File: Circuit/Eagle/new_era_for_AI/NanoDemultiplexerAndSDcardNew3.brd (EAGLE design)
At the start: 94 x 70 mm, 22 parts

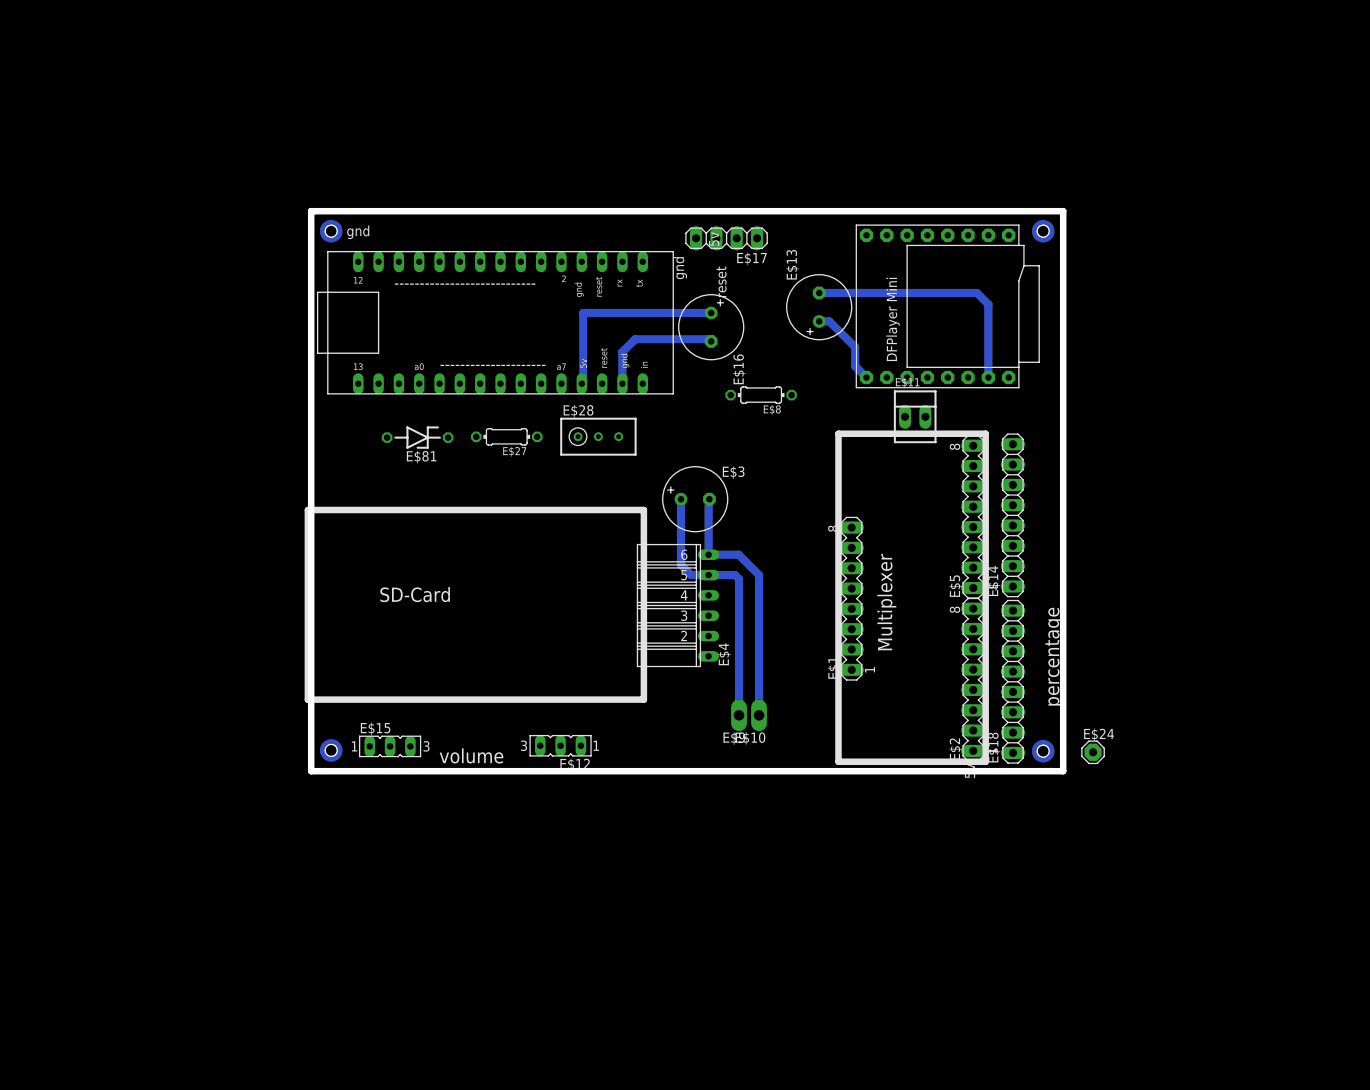
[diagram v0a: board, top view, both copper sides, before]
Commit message: .
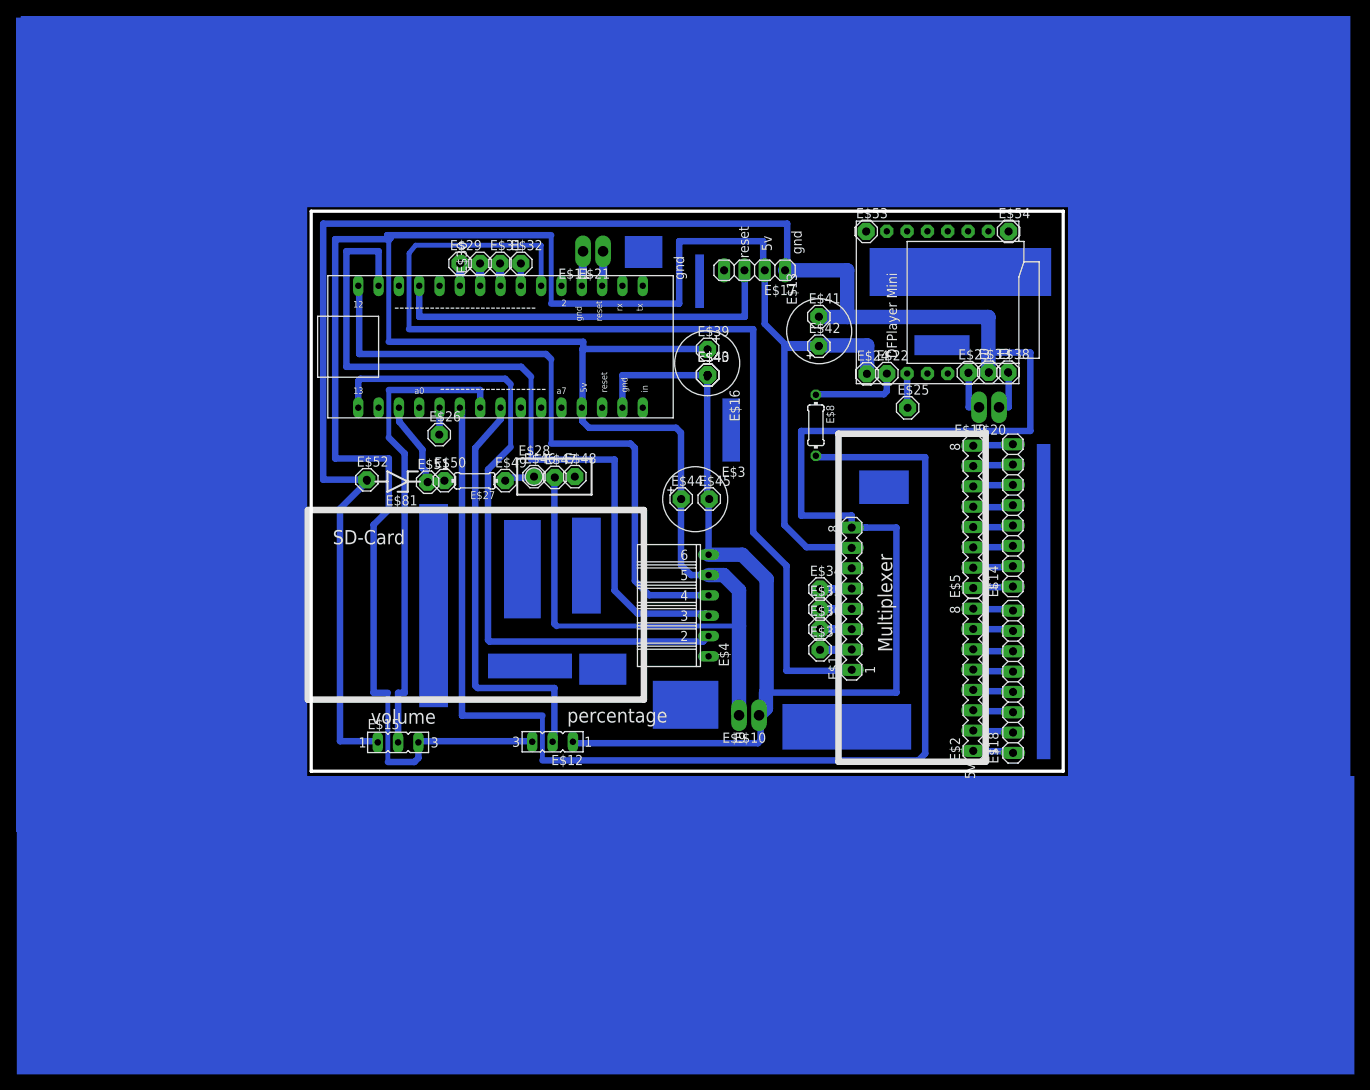
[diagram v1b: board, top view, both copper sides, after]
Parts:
- added E$19, E$20, E$21: (no value), testpad:P1-13Y
- added E$22, E$23, E$25, E$26, E$29, E$30, E$31, E$32, E$33, E$34, E$35, E$36, E$37, E$38, E$39, E$40, E$41, E$42, E$43, E$44, E$45, E$46, E$47, E$48, E$49, E$50, E$51, E$52, E$53, E$54: (no value), solpad:MCS10B
- E$11: device con-molex:22-23-2021 -> testpad:P1-13Y
- moved E$24 55.1 mm to (75.5, 51.7)
- moved E$11 46.4 mm to (40.0, 67.0), turned to 180 degrees
- moved E$8 7.81 mm to (69.1, 45.2), turned to 270 degrees
- moved E$28 7.43 mm to (36.4, 38.8)
- moved E$27 6.80 mm to (26.4, 38.3)
- moved E$81 6.04 mm to (16.8, 38.2)
- moved E$17 5.32 mm to (61.4, 64.6)
- moved E$16 4.53 mm to (55.5, 53.0)
- moved E$13 3.00 mm to (69.5, 57.0)
- moved E$7 3.00 mm to (29.7, 55.1)
- moved E$12 1.12 mm to (33.6, 5.68)
- moved E$15 1.12 mm to (19.4, 5.60)
- moved E$6 0.50 mm to (84.3, 60.6)
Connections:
- new net SPK3: E$11.TP, E$7.P$24
- new net SPK4: E$21.TP, E$7.P$25
- net S0: now also E$32.MP, E$34.MP
- net S1: now also E$31.MP, E$35.MP
- net S2: now also E$30.MP, E$36.MP
- net S3: now also E$29.MP, E$37.MP
- net SPK1: now also E$19.TP; no longer E$11.1
- net SPK2: now also E$20.TP; no longer E$11.2
- net TX: now also E$25.MP, E$26.MP
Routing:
- net 5V: track 68.4 -> 384.5 mm
- net GND: track 78.6 -> 376.8 mm
- net S$10: track 0.00 -> 153.3 mm
- net SIGN: track 0.00 -> 127.2 mm
- net MOSI: track 0.00 -> 96.6 mm
- net SCK: track 0.00 -> 83.9 mm
- net MISO: track 0.00 -> 80.6 mm
- net VOLUME-CONTROL: track 0.00 -> 59.3 mm
- net S$4: track 0.00 -> 52.8 mm
- net RESET: track 0.00 -> 50.4 mm
- net S$2: track 0.00 -> 12.7 mm
- net RX: track 0.00 -> 11.3 mm
- net TX: track 0.00 -> 7.70 mm
- net S1: track 0.00 -> 6.78 mm
- net S0: track 0.00 -> 6.77 mm
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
